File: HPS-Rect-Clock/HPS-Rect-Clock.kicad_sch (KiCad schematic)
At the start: 4 parts

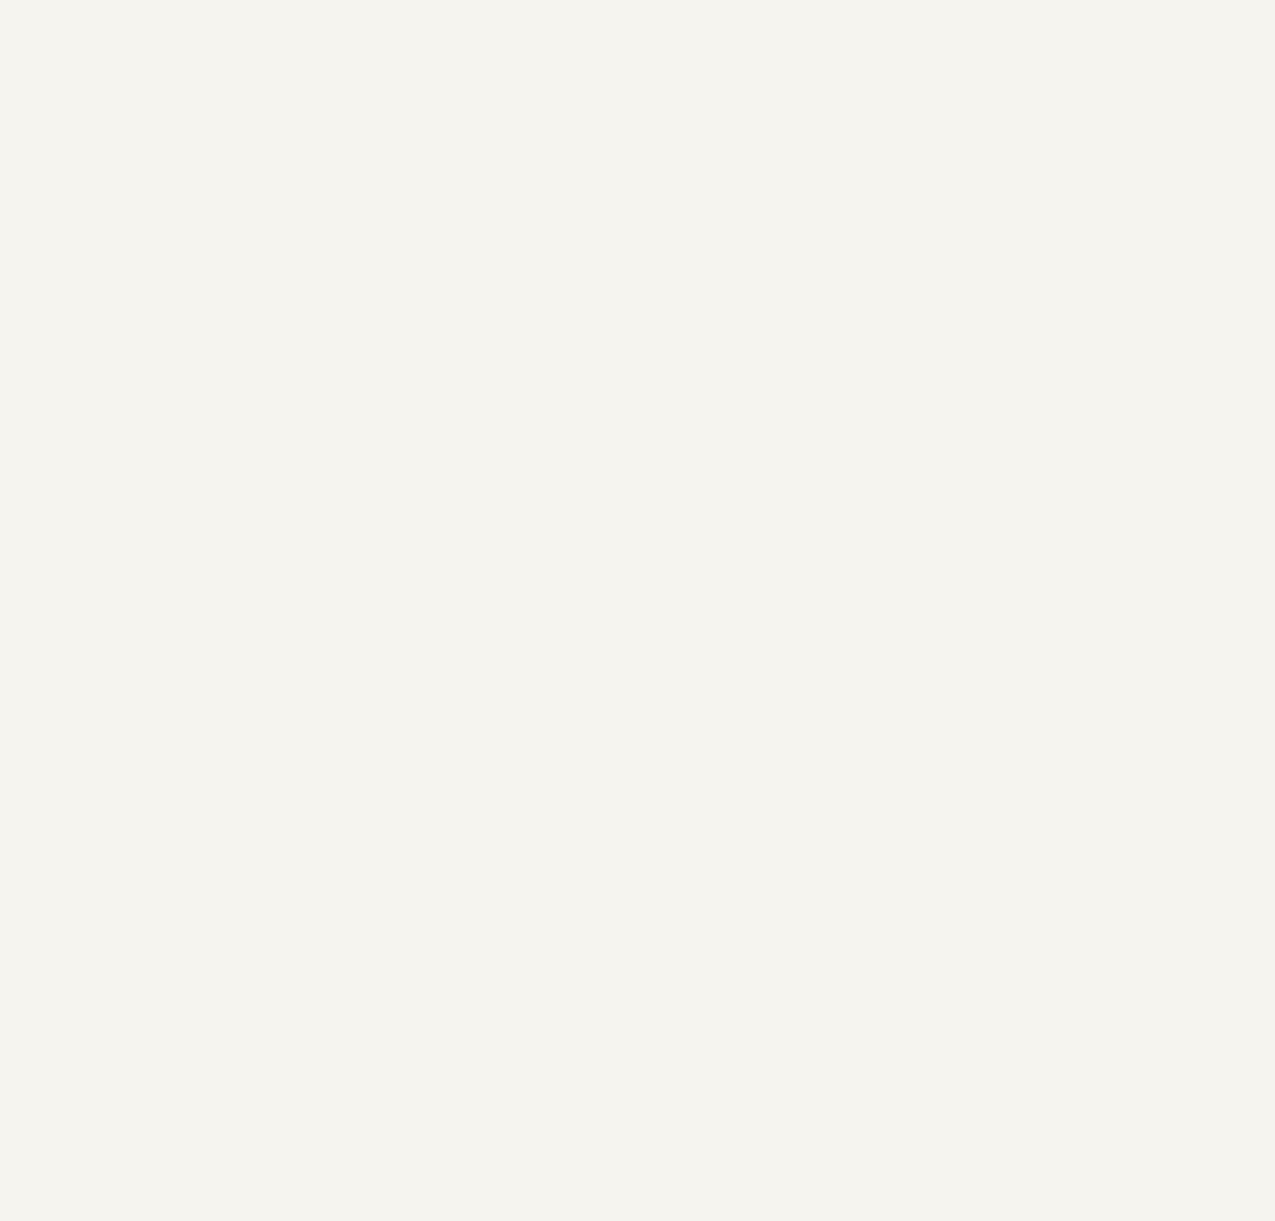
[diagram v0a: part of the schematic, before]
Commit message: Week 1 Schematics
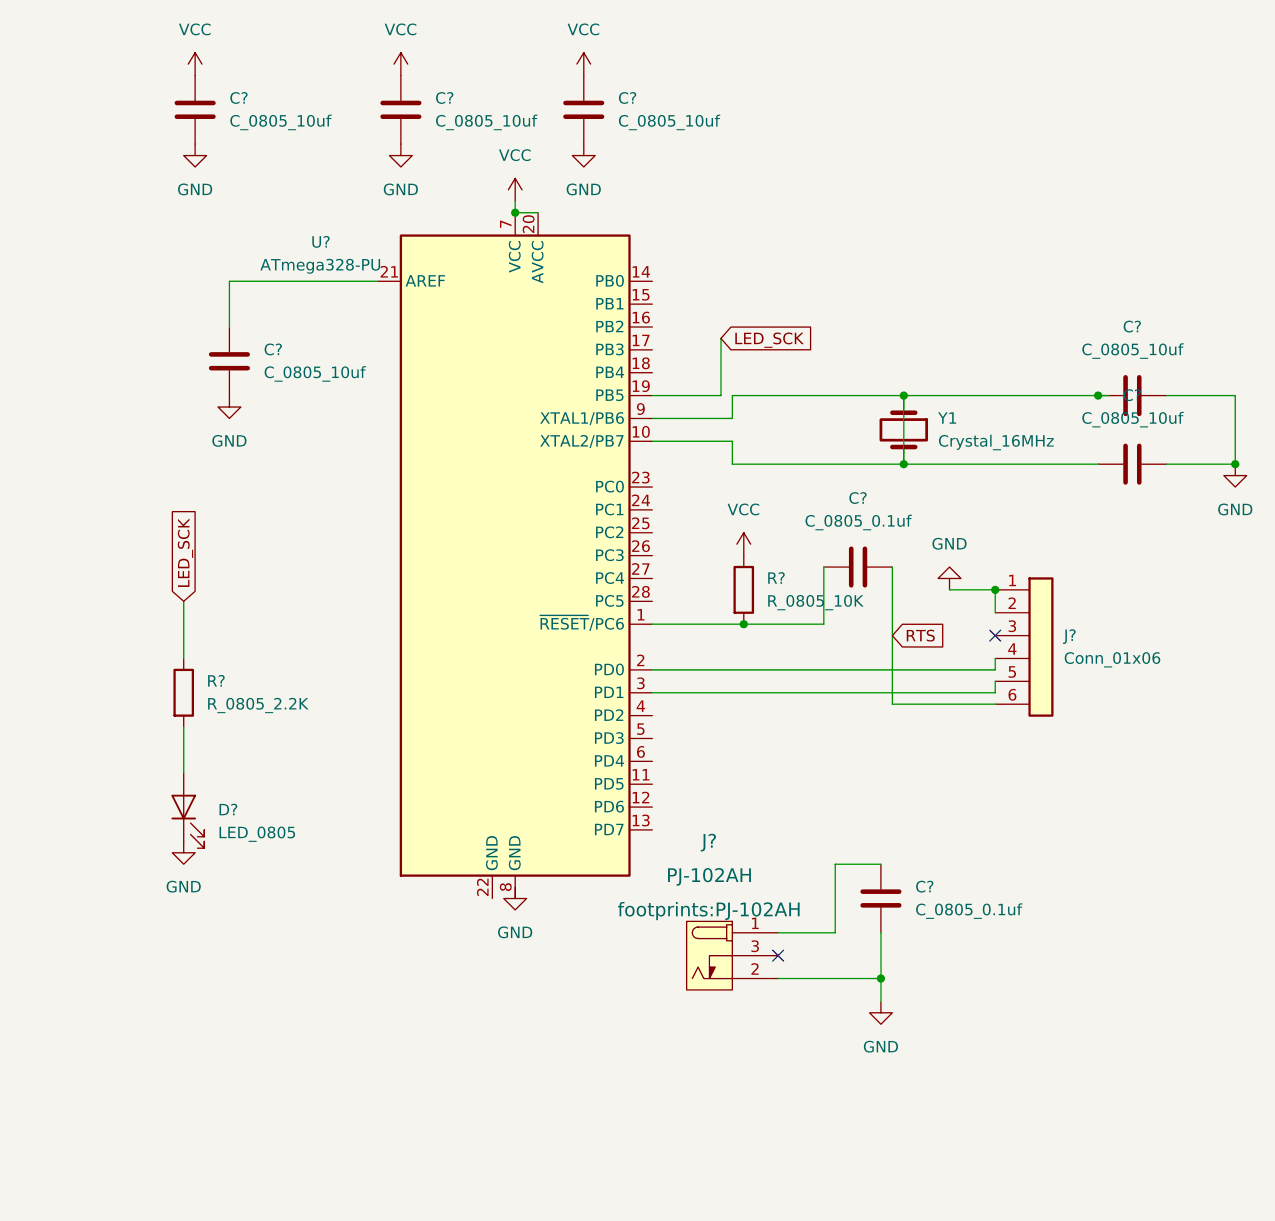
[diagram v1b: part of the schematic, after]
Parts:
- added C? (x6): C_0805_10uf, footprints:C_0805_2012Metric, symbol HPS:C_0805_10uf
- added C? (x2): C_0805_0.1uf, footprints:C_0805_2012Metric, symbol HPS:C_0805_0.1uf
- added D?: LED_0805, footprints:LED_0805_2012Metric, symbol HPS:LED_0805
- added J?: PJ-102AH, footprints:PJ-102AH, symbol HPS:PJ-102AH
- added J?: Conn_01x06, footprints:PinHeader_1x06_P2.54mm_Vertical, symbol HPS:Conn_01x06
- added R?: R_0805_2.2K, footprints:R_0805_2012Metric, symbol HPS:R_0805_2.2K
- added R?: R_0805_10K, footprints:R_0805_2012Metric, symbol HPS:R_0805_10K
- added U?: ATmega328-PU, footprints:DIP-28_W7.62mm, symbol HPS:ATmega328-PU
- added Y1: Crystal_16MHz, footprints:Crystal_SMD_HC49-SD, symbol HPS:Crystal_16MHz
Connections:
- new net: C?.2, J?.1 (POLE)
- new net: C?.1, R?.2, U?.1 (~{RESET}/PC6)
- new net: C?.1, U?.21 (AREF)
- new net: C?.1, C?.1, U?.10 (XTAL2/PB7), U?.9 (XTAL1/PB6), Y1.1, Y1.2
- new net: J?.4 (Pin_4), U?.2 (PD0)
- new net: J?.5 (Pin_5), U?.3 (PD1)
- new net: D?.2 (A), R?.2
- new net GND: C?.1, C?.2, C?.2, C?.2, C?.2, C?.2, C?.2, D?.1 (K), J?.1 (Pin_1), J?.2 (OUT), J?.2 (Pin_2)
- new net LED_SCK: R?.1, U?.19 (PB5)
- new net RTS: C?.2, J?.6 (Pin_6)
- new net VCC: C?.1, C?.1, C?.1, R?.1, U?.20 (AVCC), U?.7 (VCC)
- no-connect marks 0 -> 2

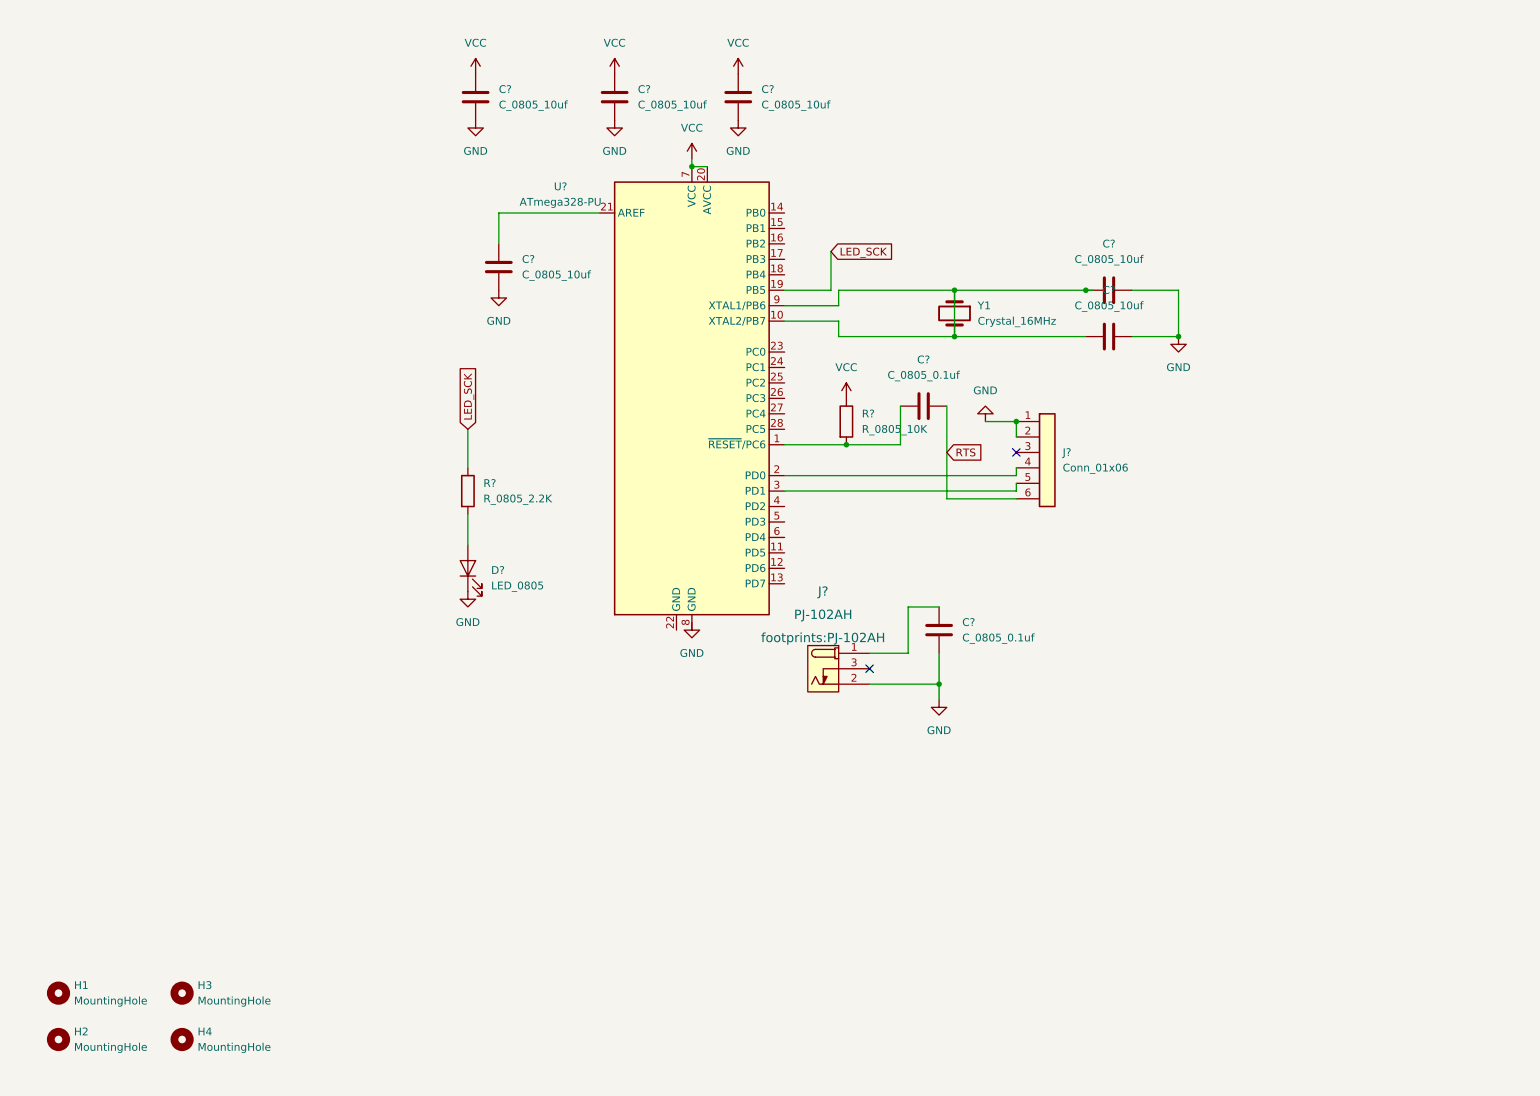
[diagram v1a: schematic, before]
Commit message: Week 2
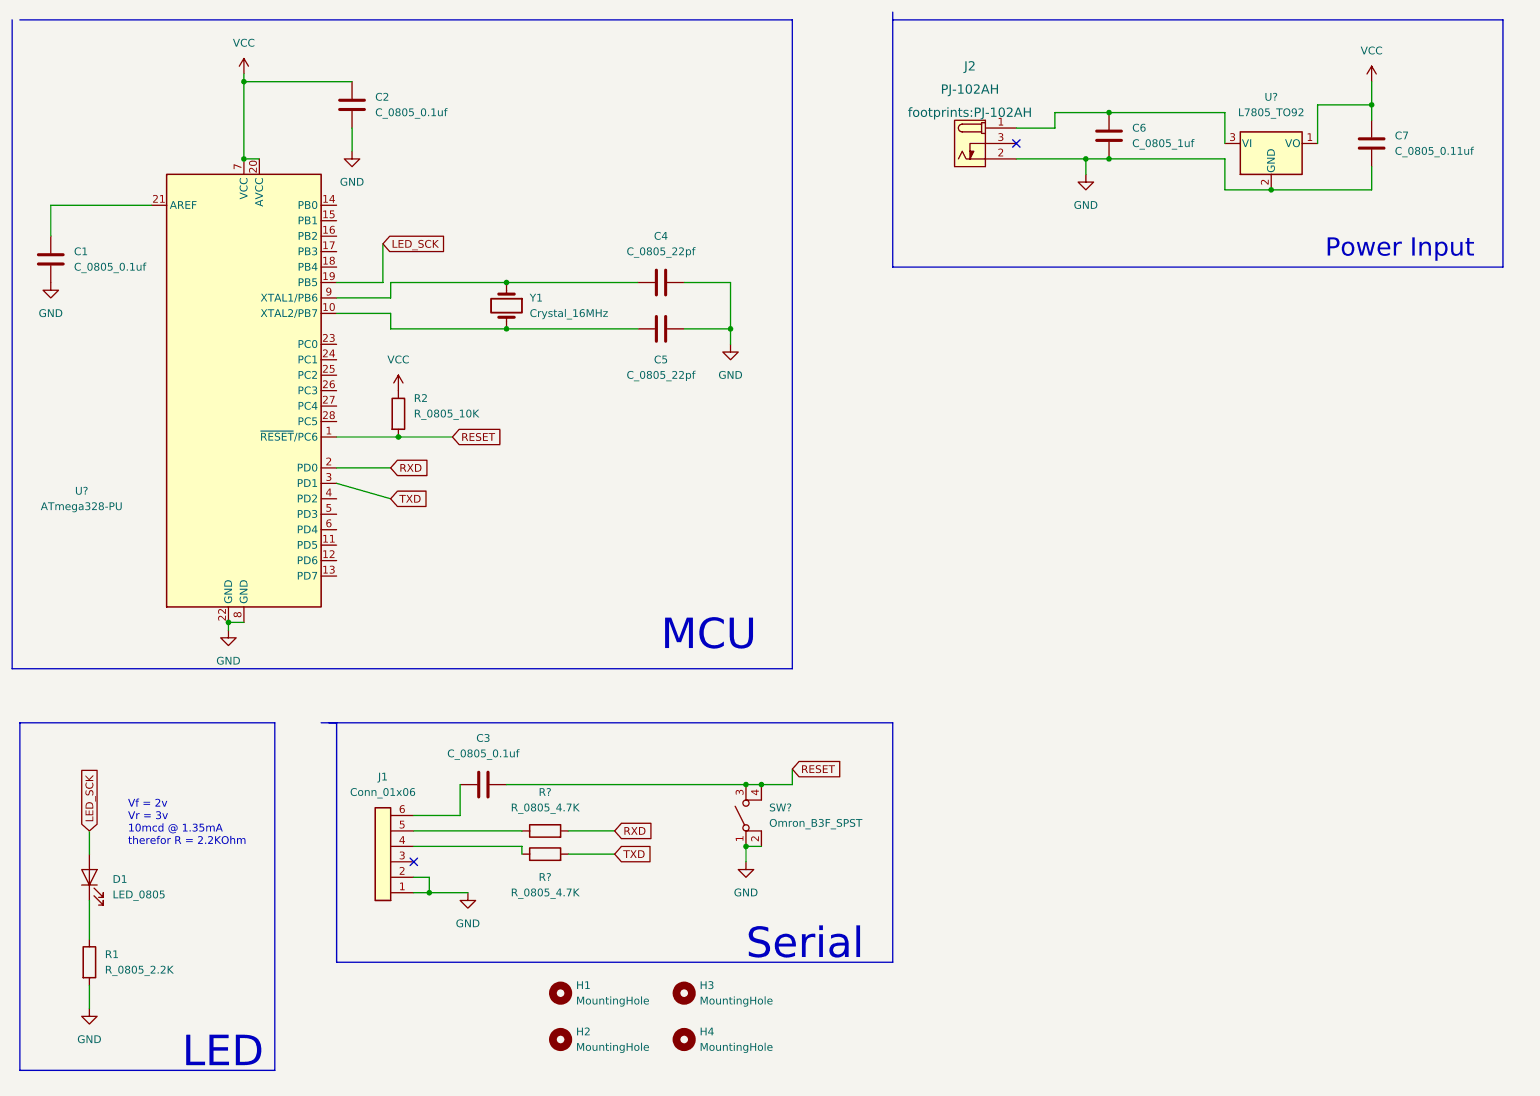
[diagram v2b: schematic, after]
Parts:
- removed C? (x3): C_0805_10uf, footprints:C_0805_2012Metric, symbol HPS:C_0805_10uf
- removed C?: C_0805_0.1uf, footprints:C_0805_2012Metric, symbol HPS:C_0805_0.1uf
- added C2: C_0805_0.1uf, footprints:C_0805_2012Metric, symbol HPS:C_0805_10uf
- added C3: C_0805_0.1uf, footprints:C_0805_2012Metric, symbol HPS:C_0805_0.1uf
- added C7: C_0805_0.11uf, footprints:C_0805_2012Metric, symbol HPS:C_0805_0.1uf
- added R? (x2): R_0805_4.7K, footprints:R_0805_2012Metric, symbol HPS:R_0805_4.7K
- added SW?: Omron_B3F_SPST, footprints:SW_SPST_Omron_B3FS-100xP, symbol HPS:Omron_B3F_SPST
- added U?: L7805_TO92, footprints:TO-92_Inline, symbol HPS:L7805_TO92
- C1: renamed from C?; value C_0805_10uf -> C_0805_0.1uf
- C4, C5: renamed from C?; value C_0805_10uf -> C_0805_22pf
- C6: renamed from C?; value C_0805_0.1uf -> C_0805_1uf
- gave numbers to parts that had none: 5
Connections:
- net GND: now also R1.2, U?.22 (GND), U?.8 (GND), C2.2, C7.1, SW?.1 (A), SW?.2 (A), U?.2 (GND); no longer D1.1 (K)
- net LED_SCK: now also D1.2 (A); no longer R1.1
- net VCC: now also C2.1, C7.2, U?.1 (VO)
- net at C6.2, J2.1 (POLE): now also U?.3 (VI)
- net RESET: now reaches R2.2, U?.1 (~{RESET}/PC6)
- net RESET: now also C3.1, SW?.3 (B), SW?.4 (B)
- net at C4.1, U?.9 (XTAL1/PB6), Y1.1: no longer C5.1, U?.10 (XTAL2/PB7), Y1.2
- net at J1.4 (Pin_4): now also R?.1; no longer U?.2 (PD0)
- net at J1.5 (Pin_5): now also R?.1; no longer U?.3 (PD1)
- net RTS: no longer names the net of J1.6 (Pin_6)
- net RTS: now also C3.2
- new net: C5.1, U?.10 (XTAL2/PB7), Y1.2
- new net: D1.1 (K), R1.1
- new net RXD: R?.2, U?.2 (PD0)
- new net TXD: R?.2, U?.3 (PD1)
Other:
- note added: "LED"
- note added: "MCU"
- note added: "Power Input"
- note added: "Serial"
- note added: "Vf = 2v Vr = 3v 10mcd @ 1.35mA therefor R = 2.2KOhm"
- moved on the sheet: C1, C4, C5, C6, D1, H1, H2, H3, H4, J1, J2, R1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
